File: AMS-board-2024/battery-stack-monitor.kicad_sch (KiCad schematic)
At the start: 68 parts, among them Q115 STD7ANM60N, Q116 2N7002K-AU, Q117 STD7ANM60N, Q118 STD7ANM60N, U23 LM25180-Q1, U24 NCV8711BMTW500TBG, U25 LTC2949, U26 NV24C16SNVLT3G, Y2 ABLS-4.000MHZ-K4T

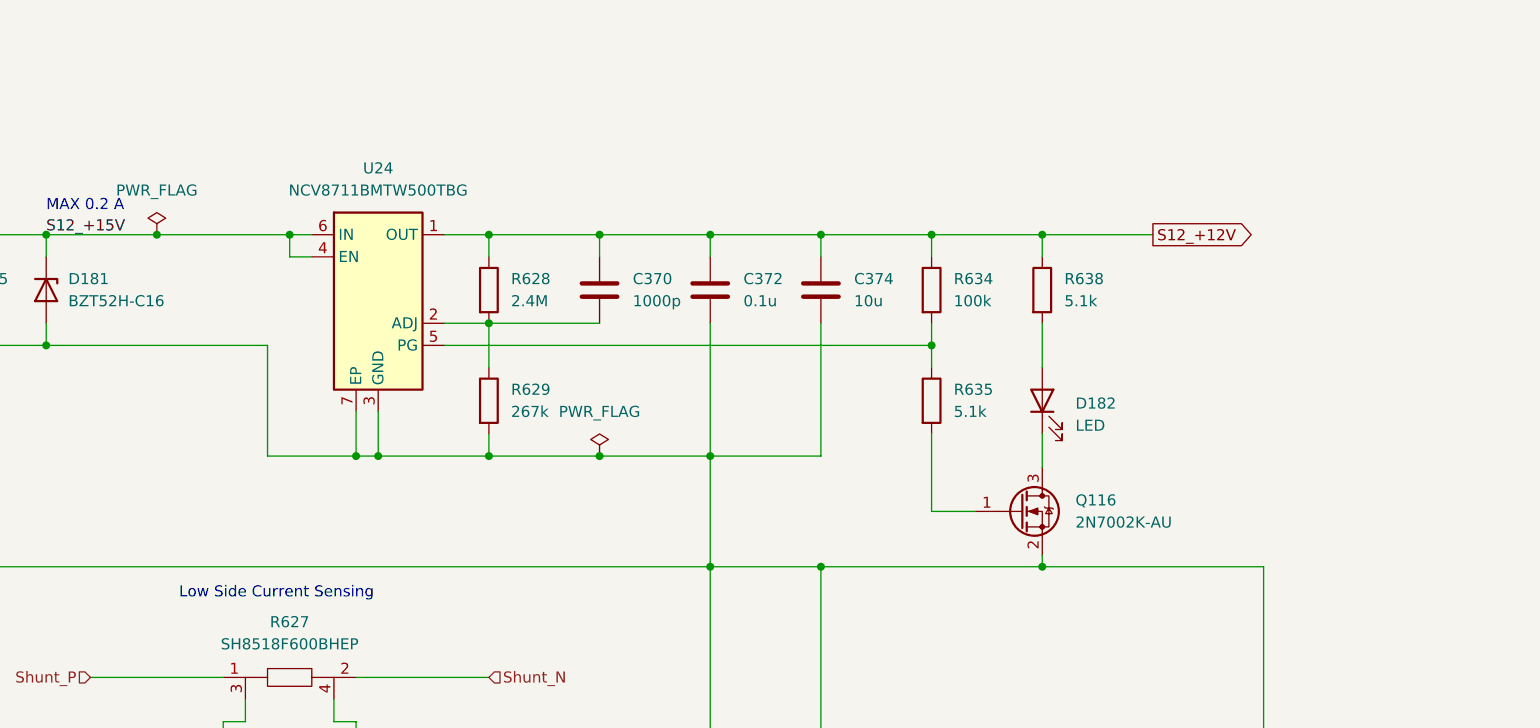
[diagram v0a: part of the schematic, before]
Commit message: リニアレギュレータの入力にコンデンサを追加
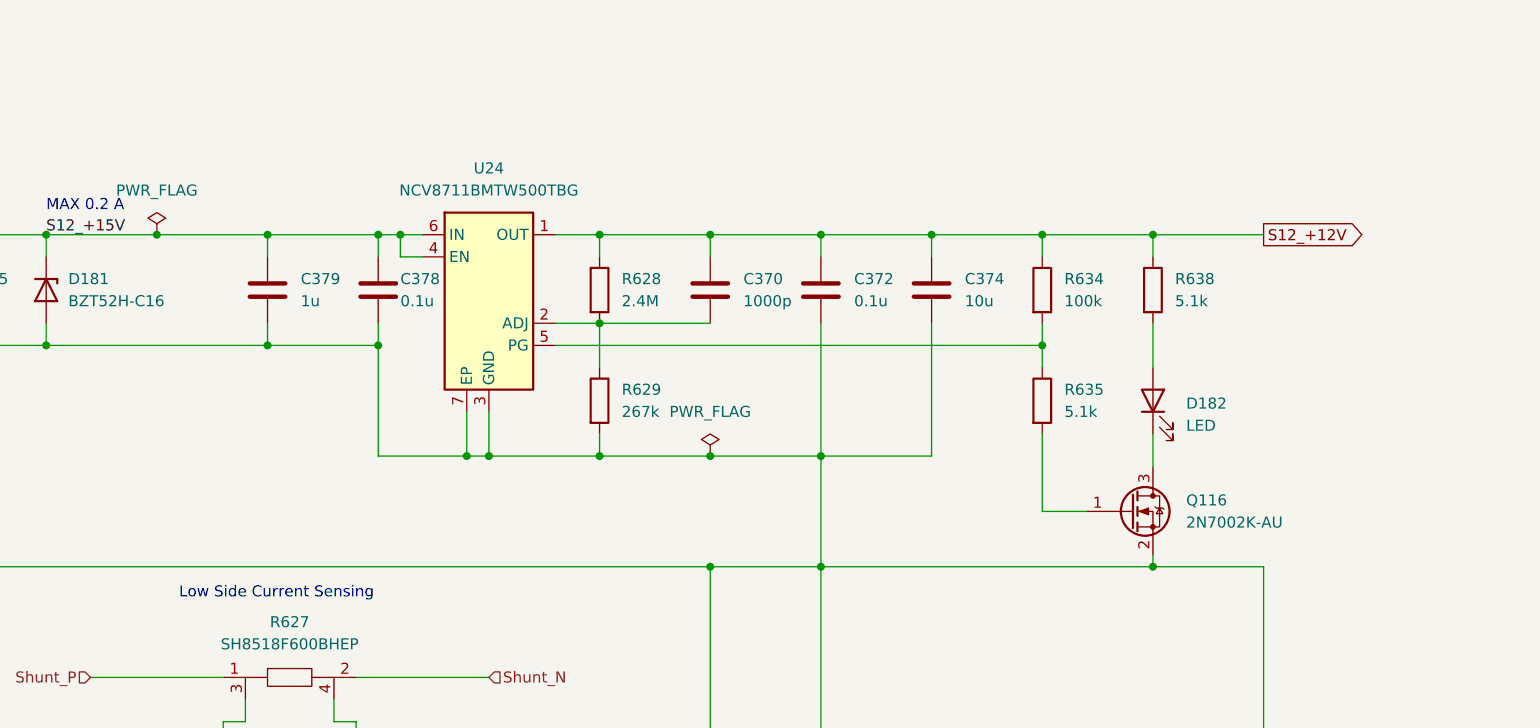
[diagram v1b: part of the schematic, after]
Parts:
- added C378: 0.1u, Capacitor_SMD:C_0402_1005Metric, symbol Device:C
- added C379: 1u, Capacitor_SMD:C_0402_1005Metric, symbol Device:C
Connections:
- net S12_+15V: now also C378.1, C379.1
- net V_{ACC}-: now also C378.2, C379.2
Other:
- moved on the sheet: C370, C372, C374, D182, Q116, R628, R629, R634, R635, R638, U24

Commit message: 2M Ohmsのチップ抵抗のサイズを3216に変更
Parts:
- R632, R639, R643: footprint Resistor_SMD:R_0603_1608Metric -> Resistor_SMD:R_1206_3216Metric
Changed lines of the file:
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@@
       (effects (font (size 1.27 1.27)) (justify right))
     )
-    (property "Footprint" "Resistor_SMD:R_0603_1608Metric" (at 255.778 222.25 90)
+    (property "Footprint" "Resistor_SMD:R_1206_3216Metric" (at 255.778 222.25 90)
       (effects (font (size 1.27 1.27)) hide)
     )
@@
       (effects (font (size 1.27 1.27)) (justify right))
     )
-    (property "Footprint" "Resistor_SMD:R_0603_1608Metric" (at 293.878 196.85 90)
+    (property "Footprint" "Resistor_SMD:R_1206_3216Metric" (at 293.878 196.85 90)
       (effects (font (size 1.27 1.27)) hide)
     )
@@
       (effects (font (size 1.27 1.27)) (justify right))
     )
-    (property "Footprint" "Resistor_SMD:R_0603_1608Metric" (at 331.978 196.85 90)
-      (effects (font (size 1.27 1.27)) hide)
-    )
+    (property "Footprint" "Resistor_SMD:R_1206_3216Metric" (at 331.978 196.85 90)
+      (effects (font (size 1.27 1.27)) hide)
+    )
